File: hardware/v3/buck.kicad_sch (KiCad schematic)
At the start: 44 parts, among them J1 Conn_01x02_Pin, J6 Conn_01x03_Pin, Q1 C3M0030090K, Q2 C3M0030090K, Q4 T2N7002AK, U10 H11L1, U12 SN74LVC2G14DBV, U13 MCP9501PT-065E/OT, U14 74AHC1G02, U16 MCP6022, U17 LM555xM, U18 MCP6561-OT, U5 UCC5350MCQDRQ1, U6 MCP9501PT-065E/OT, U7 UCC5350MCQDRQ1, U9 LM5106SD

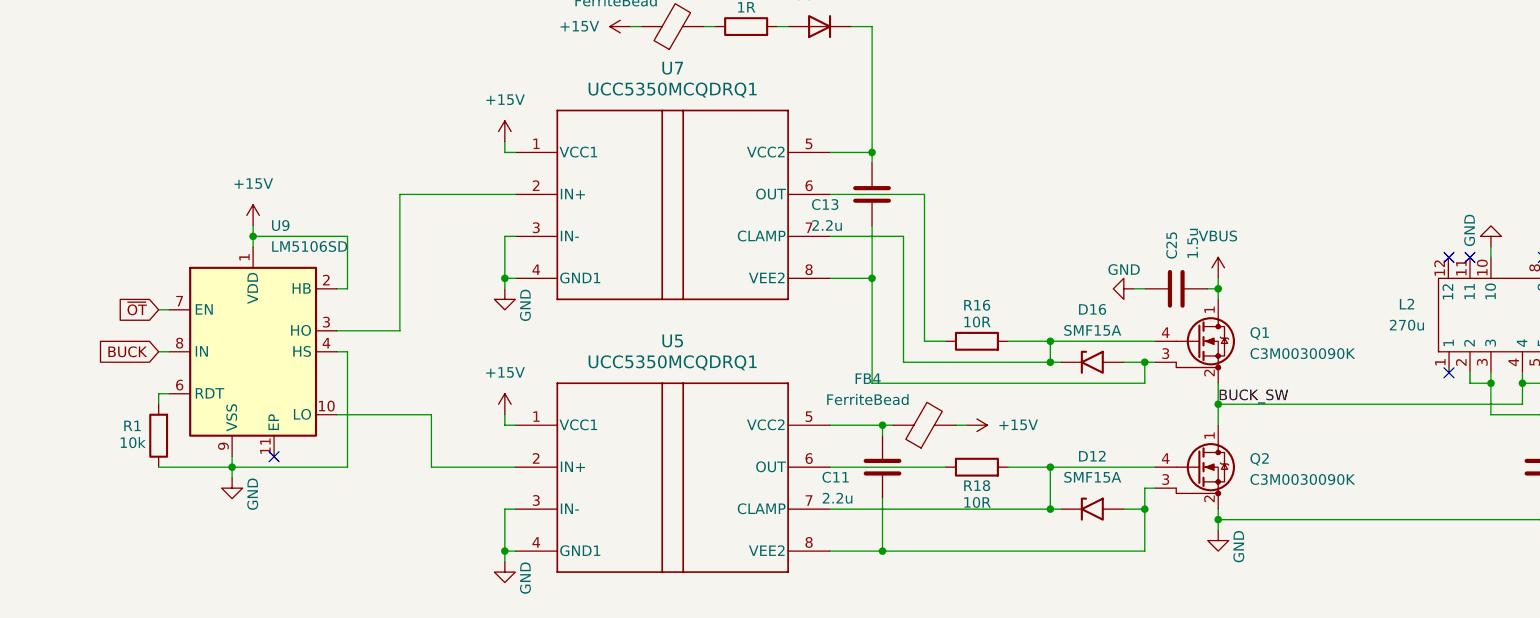
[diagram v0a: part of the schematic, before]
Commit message: ?
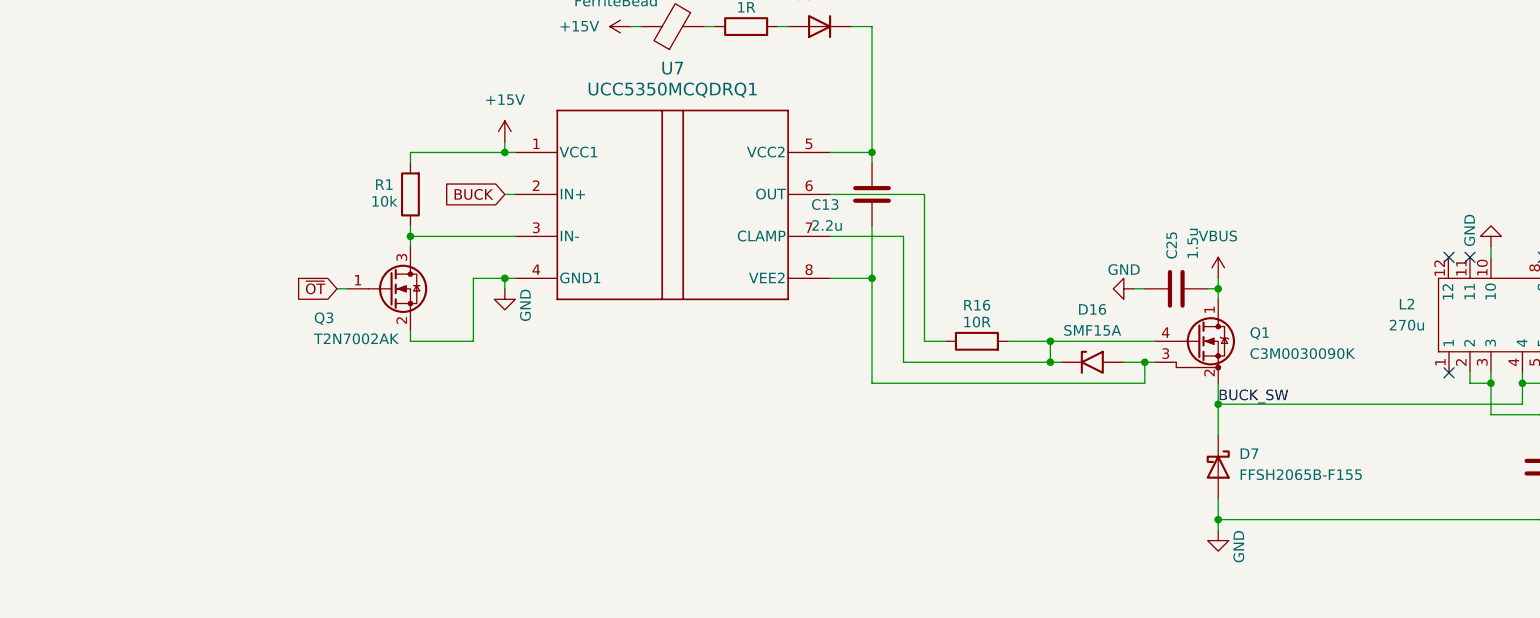
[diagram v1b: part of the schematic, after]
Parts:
- removed C11: 2.2u, Capacitor_SMD:C_0805_2012Metric, symbol Device:C
- removed D12: SMF15A, Diode_SMD:D_SMF, symbol Diode:SMF15A
- removed FB4: FerriteBead, Inductor_SMD:L_0805_2012Metric, symbol Device:FerriteBead
- removed Q2: C3M0030090K, Package_TO_SOT_THT:TO-247-4_Horizontal_TabUp, symbol Transistor_FET:C3M0030090K
- removed R18: 10R, Resistor_SMD:R_0805_2012Metric, symbol Device:R
- removed U5: UCC5350MCQDRQ1, Package_SO:SOIC-8_3.9x4.9mm_P1.27mm, symbol New_Library:UCC5350MCQDRQ1
- removed U9: LM5106SD, Package_SO:VSSOP-10_3x3mm_P0.5mm, symbol Driver_FET:LM5106SD
- added D7: FFSH2065B-F155, Package_TO_SOT_THT:TO-247-2_Horizontal_TabUp, symbol Diode:C3D25170H
- added Q3: T2N7002AK, Package_TO_SOT_SMD:SOT-23, symbol Transistor_FET:T2N7002AK
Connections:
- net +15V: now also R1.2
- net BUCK: now also U7.2 (IN+)
- net BUCK_SW: now also D7.1 (K)
- net GND: now also D7.2 (A), Q3.2 (S); no longer R1.1, U7.3 (IN-)
- net ~{OT}: now also Q3.1 (G)
- new net: Q3.3 (D), R1.1, U7.3 (IN-)
- no-connect marks 9 -> 8
